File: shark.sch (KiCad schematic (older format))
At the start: 125 parts, among them J1 USB_B, SW1 MXSwitch, SW10 MXSwitch, SW11 MXSwitch, SW12 MXSwitch, SW13 MXSwitch, SW14 MXSwitch, SW15 MXSwitch, SW16 MXSwitch, SW17 MXSwitch, SW18 MXSwitch, SW19 MXSwitch, SW2 MXSwitch, SW20 MXSwitch, SW21 MXSwitch, SW22 MXSwitch, SW23 MXSwitch, SW24 MXSwitch, SW25 MXSwitch, SW26 MXSwitch, SW27 MXSwitch, SW28 MXSwitch, SW29 MXSwitch, SW3 MXSwitch, SW30 MXSwitch, SW31 MXSwitch, SW32 MXSwitch, SW33 MXSwitch, SW34 MXSwitch, SW35 MXSwitch, SW36 MXSwitch, SW37 MXSwitch, SW38 MXSwitch, SW39 MXSwitch, SW4 MXSwitch, SW40 MXSwitch, SW41 MXSwitch, SW42 MXSwitch, SW43 MXSwitch, SW44 MXSwitch, SW45 MXSwitch, SW46 MXSwitch, SW47 MXSwitch, SW48 MXSwitch, SW49 MXSwitch, SW5 MXSwitch, SW50 MXSwitch, SW51 MXSwitch, SW6 MXSwitch, SW7 MXSwitch, SW8 MXSwitch, SW9 MXSwitch, U1 ATmega32U4-AU, Y1 Crystal

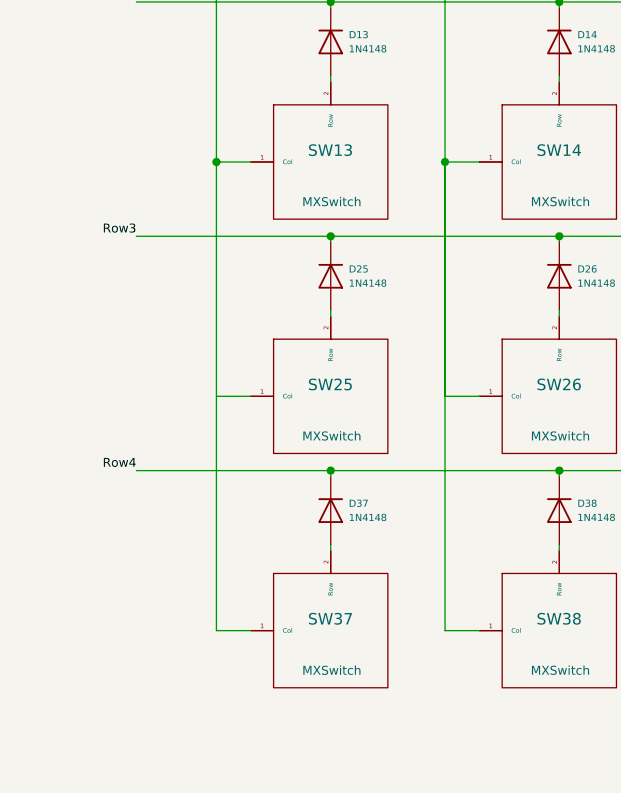
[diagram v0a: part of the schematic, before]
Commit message: Added row and column traces, fixed some components positions
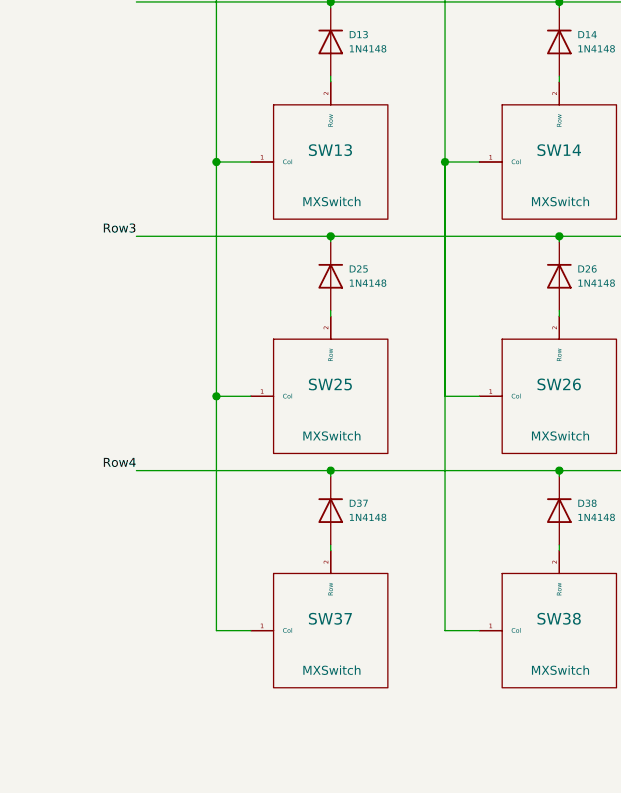
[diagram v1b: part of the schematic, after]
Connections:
- net Col1: now also SW25.1 (Col)
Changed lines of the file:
@@
 $EndComp
 Wire Wire Line
-	2150 3725 2150 5775
+	2150 3725 2150 4750
 Wire Wire Line
 	2150 2700 2150 3725
@@
 Wire Wire Line
 	6650 6100 6950 6100
+Connection ~ 2150 4750
+Wire Wire Line
+	2150 4750 2150 5775
 $EndSCHEMATC

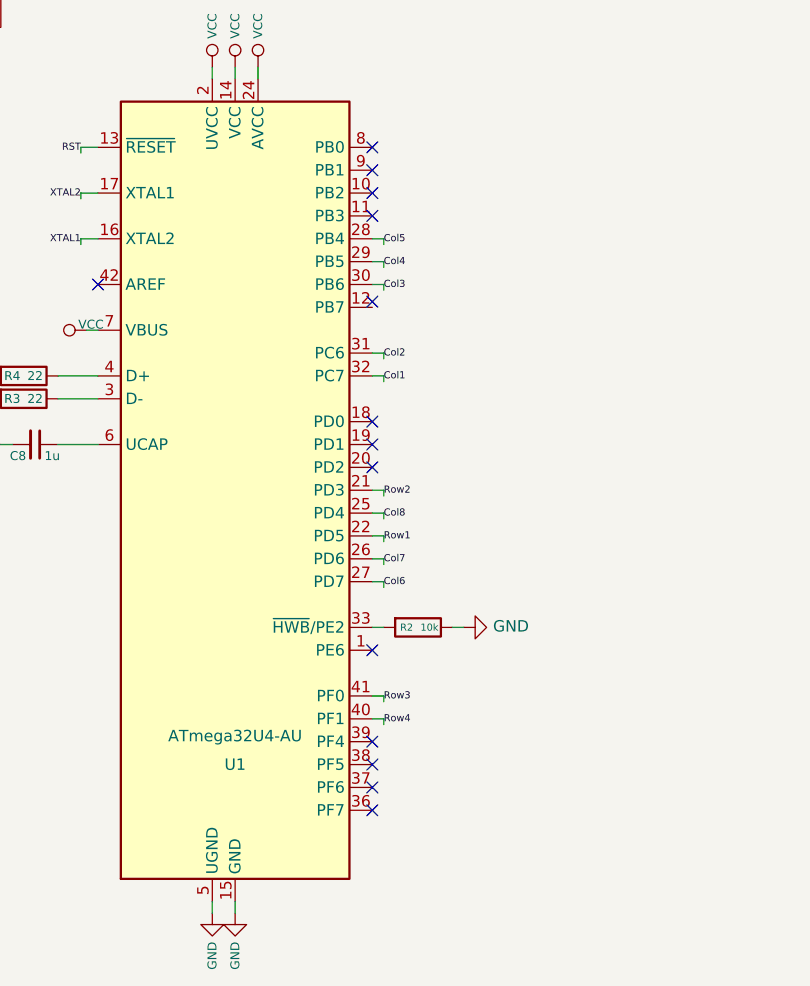
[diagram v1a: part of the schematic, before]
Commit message: Continued tracing
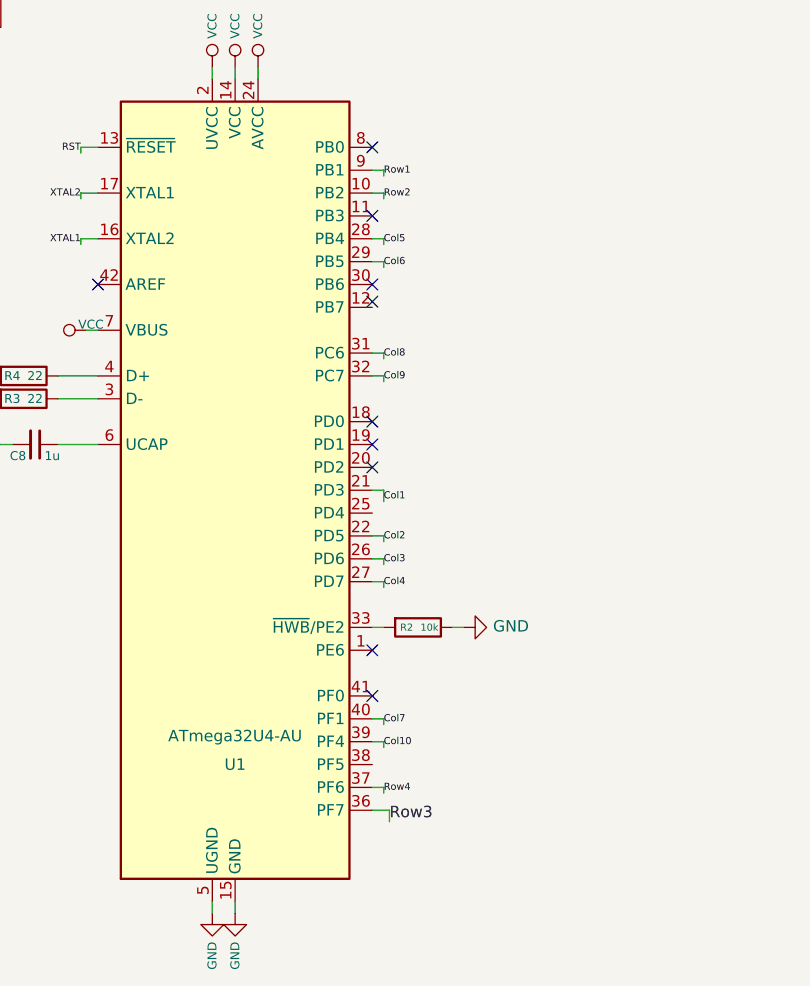
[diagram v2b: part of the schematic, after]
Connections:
- net Col1: now also U1.21 (PD3); no longer U1.32 (PC7)
- net Col10: now also U1.39 (PF4)
- net Col2: now also U1.22 (PD5); no longer U1.31 (PC6)
- net Col3: now also U1.26 (PD6); no longer U1.30 (PB6)
- net Col4: now also U1.27 (PD7); no longer U1.29 (PB5)
- net Col6: now also U1.29 (PB5); no longer U1.27 (PD7)
- net Col7: now also U1.40 (PF1); no longer U1.26 (PD6)
- net Col8: now also U1.31 (PC6); no longer U1.25 (PD4)
- net Col9: now also U1.32 (PC7)
- net Row1: now also U1.9 (PB1); no longer U1.22 (PD5)
- net Row2: now also U1.10 (PB2); no longer U1.21 (PD3)
- net Row3: now also U1.36 (PF7); no longer U1.41 (PF0)
- net Row4: now also U1.37 (PF6); no longer U1.40 (PF1)
- no-connect marks 14 -> 10
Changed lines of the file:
@@
 	10575 9400 10525 9400
-$Comp
-L power:GND #PWR0107
-U 1 1 5BEE37FA
-P 2125 8975
-F 0 "#PWR0107" H 2125 8725 50  0001 C CNN
-F 1 "GND" V 2130 8847 50  0000 R CNN
-F 2 "" H 2125 8975 50  0001 C CNN
-F 3 "" H 2125 8975 50  0001 C CNN
-	1    2125 8975
-	1    0    0    -1
-$EndComp
 $Comp
 L power:GND #PWR0108
@@
 Wire Wire Line
 	2225 8925 2225 9075
-Wire Wire Line
-	2125 8925 2125 8975
 $Comp
 L Device:R R3
@@
 	9250 7300 9325 7300
 Wire Wire Line
-	10525 8800 10575 8800
-Wire Wire Line
-	10525 9000 10575 9000
-Text Label 10575 8825 0    31   ~ 0
+	10525 7500 10575 7500
+Wire Wire Line
+	10525 7400 10575 7400
+Text Label 10575 7525 0    31   ~ 0
 Row2
-Text Label 10575 9025 0    31   ~ 0
+Text Label 10575 7425 0    31   ~ 0
 Row1
 Wire Wire Line
-	10525 8900 10575 8900
-Wire Wire Line
 	10525 9100 10575 9100
 Wire Wire Line
+	10525 9800 10575 9800
+Wire Wire Line
 	10525 9200 10575 9200
 Wire Wire Line
@@
 Wire Wire Line
 	10525 7800 10575 7800
-Wire Wire Line
-	10525 7900 10575 7900
-Text Label 10575 8925 0    31   ~ 0
-Col8
 Text Label 10575 9125 0    31   ~ 0
+Col3
+Text Label 10575 9825 0    31   ~ 0
 Col7
 Text Label 10575 9225 0    31   ~ 0
-Col6
+Col4
 Text Label 10575 7725 0    31   ~ 0
 Col5
 Text Label 10575 7825 0    31   ~ 0
-Col4
-Text Label 10575 7925 0    31   ~ 0
-Col3
-Wire Wire Line
-	10575 7925 10575 7900
+Col6
 Wire Wire Line
 	10575 7825 10575 7800
@@
 	10575 9200 10575 9225
 Wire Wire Line
+	10575 9800 10575 9825
+Wire Wire Line
 	10575 9100 10575 9125
-Wire Wire Line
-	10575 8900 10575 8925
 NoConn ~ 10525 9500
 Wire Wire Line
@@
 	10575 8300 10575 8325
 Text Label 10575 8325 0    31   ~ 0
-Col1
+Col9
 Text Label 10575 8225 0    31   ~ 0
-Col2
-Wire Wire Line
-	10525 9800 10575 9800
-Wire Wire Line
-	10575 9800 10575 9825
-Wire Wire Line
-	10525 9700 10575 9700
-Wire Wire Line
-	10575 9700 10575 9725
-Text Label 10575 9725 0    31   ~ 0
-Row3
-Text Label 10575 9825 0    31   ~ 0
+Col8
+Wire Wire Line
+	10525 10100 10575 10100
+Wire Wire Line
+	10575 10100 10575 10125
+Text Label 10575 10125 0    31   ~ 0
 Row4
 $Comp
@@
 $EndComp
 NoConn ~ 10525 7300
-NoConn ~ 10525 7400
-NoConn ~ 10525 7500
 NoConn ~ 10525 7600
 NoConn ~ 10525 7975
@@
 NoConn ~ 10525 8700
 Wire Wire Line
-	10575 9000 10575 9025
-Wire Wire Line
-	10575 8800 10575 8825
-NoConn ~ 10525 10200
-NoConn ~ 10525 10100
-NoConn ~ 10525 10000
-NoConn ~ 10525 9900
+	10575 7400 10575 7425
+Wire Wire Line
+	10575 7500 10575 7525
 NoConn ~ 9325 7900
 $Comp
@@
 Wire Wire Line
 	2150 4750 2150 5775
+Wire Wire Line
+	2125 8925 2125 8975
+$Comp
+L power:GND #PWR0107
+U 1 1 5BEE37FA
+P 2125 8975
+F 0 "#PWR0107" H 2125 8725 50  0001 C CNN
+F 1 "GND" V 2130 8847 50  0000 R CNN
+F 2 "" H 2125 8975 50  0001 C CNN
+F 3 "" H 2125 8975 50  0001 C CNN
+	1    2125 8975
+	1    0    0    -1
+$EndComp
+Wire Wire Line
+	10525 10200 10600 10200
+Wire Wire Line
+	10600 10200 10600 10250
+Text Label 10600 10250 0    50   ~ 0
+Row3
+NoConn ~ 10525 9700
+Wire Wire Line
+	10525 9900 10575 9900
+Wire Wire Line
+	10575 9900 10575 9925
+Text Label 10575 9925 0    31   ~ 0
+Col10
+NoConn ~ 10525 7900
+Wire Wire Line
+	10525 9000 10575 9000
+Text Label 10575 9025 0    31   ~ 0
+Col2
+Wire Wire Line
+	10575 9000 10575 9025
+Wire Wire Line
+	10525 8800 10575 8800
+Wire Wire Line
+	10575 8800 10575 8850
+Text Label 10575 8850 0    31   ~ 0
+Col1
 $EndSCHEMATC

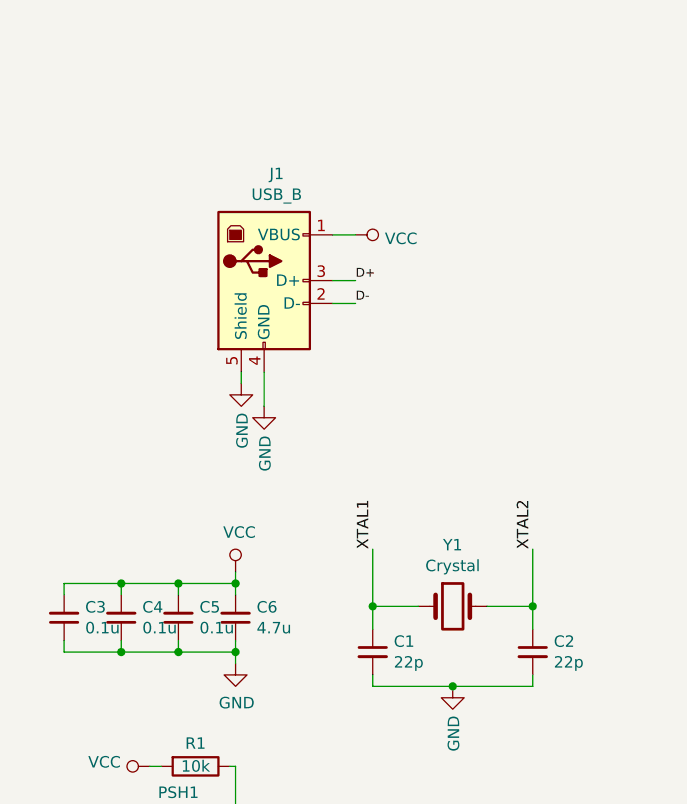
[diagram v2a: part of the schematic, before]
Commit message: Finished routing
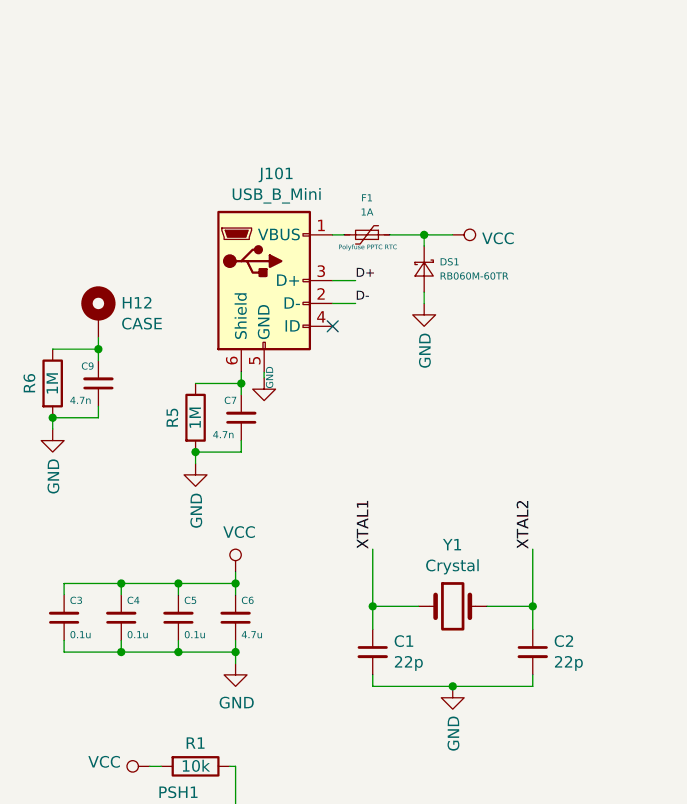
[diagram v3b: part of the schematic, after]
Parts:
- removed J1: USB_B, Connector_USB:USB_Micro-B_GCT_USB3076-30-A, symbol Connector:USB_B
- added C7, C9: 4.7n, Capacitor_SMD:C_0805_2012Metric_Pad1.15x1.40mm_HandSolder, symbol Device:C_Small
- added DS1: RB060M-60TR, Diode_SMD:D_SOD-123, symbol Device:D_Schottky_Small
- added F1: 1A, Fuse:Fuse_0805_2012Metric_Pad1.15x1.40mm_HandSolder, symbol Device:Polyfuse_Small
- added H12: CASE, Connector_Pin:Pin_D1.0mm_L10.0mm, symbol Mechanical:MountingHole_Pad
- added J101: USB_B_Mini, Keyboard_switches:miniB_connector, symbol Connector:USB_B_Mini
- added R5, R6: 1M, Resistor_SMD:R_1206_3216Metric_Pad1.42x1.75mm_HandSolder, symbol Device:R
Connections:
- net D+: now also J101.3 (D+)
- net D-: now also J101.2 (D-)
- net GND: now also C7.1, C9.1, DS1.2 (A), J101.5 (GND), R5.2, R6.2
- net VCC: now also DS1.1 (K), F1.1
- new net: C7.2, J101.6 (Shield), R5.1
- new net: F1.2, J101.1 (VBUS)
- new net: C9.2, H12.1, R6.1
- no-connect marks 10 -> 11
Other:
- note added: "Polyfuse PPTC RTC"
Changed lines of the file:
@@
 U 1 1 5BEDC719
 P 1350 10000
-F 0 "C3" H 1258 9954 50  0000 R CNN
-F 1 "0.1u" H 1258 10045 50  0000 R CNN
+F 0 "C3" H 1325 9925 31  0000 R CNN
+F 1 "0.1u" H 1325 10075 31  0000 R CNN
 F 2 "Capacitor_SMD:C_0805_2012Metric_Pad1.15x1.40mm_HandSolder" H 1350 10000 50  0001 C CNN
 F 3 "~" H 1350 10000 50  0001 C CNN
@@
 U 1 1 5BEDCA86
 P 1600 10000
-F 0 "C4" H 1508 9954 50  0000 R CNN
-F 1 "0.1u" H 1508 10045 50  0000 R CNN
+F 0 "C4" H 1575 9925 31  0000 R CNN
+F 1 "0.1u" H 1575 10075 31  0000 R CNN
 F 2 "Capacitor_SMD:C_0805_2012Metric_Pad1.15x1.40mm_HandSolder" H 1600 10000 50  0001 C CNN
 F 3 "~" H 1600 10000 50  0001 C CNN
@@
 U 1 1 5BEDCAA4
 P 1850 10000
-F 0 "C5" H 1758 9954 50  0000 R CNN
-F 1 "0.1u" H 1758 10045 50  0000 R CNN
+F 0 "C5" H 1825 9925 31  0000 R CNN
+F 1 "0.1u" H 1825 10075 31  0000 R CNN
 F 2 "Capacitor_SMD:C_0805_2012Metric_Pad1.15x1.40mm_HandSolder" H 1850 10000 50  0001 C CNN
 F 3 "~" H 1850 10000 50  0001 C CNN
@@
 U 1 1 5BEDCAC4
 P 2100 10000
-F 0 "C6" H 2008 9954 50  0000 R CNN
-F 1 "4.7u" H 2008 10045 50  0000 R CNN
+F 0 "C6" H 2075 9925 31  0000 R CNN
+F 1 "4.7u" H 2075 10075 31  0000 R CNN
 F 2 "Capacitor_SMD:C_0805_2012Metric_Pad1.15x1.40mm_HandSolder" H 2100 10000 50  0001 C CNN
 F 3 "~" H 2100 10000 50  0001 C CNN
@@
 L power:GND #PWR0108
 U 1 1 5BEE3841
-P 2225 9075
-F 0 "#PWR0108" H 2225 8825 50  0001 C CNN
-F 1 "GND" V 2230 8947 50  0000 R CNN
-F 2 "" H 2225 9075 50  0001 C CNN
-F 3 "" H 2225 9075 50  0001 C CNN
-	1    2225 9075
+P 2225 8950
+F 0 "#PWR0108" H 2225 8700 50  0001 C CNN
+F 1 "GND" V 2250 9000 31  0000 R CNN
+F 2 "" H 2225 8950 50  0001 C CNN
+F 3 "" H 2225 8950 50  0001 C CNN
+	1    2225 8950
 	1    0    0    -1
 $EndComp
@@
 Wire Wire Line
 	2625 8625 2525 8625
-Wire Wire Line
-	2625 8325 2525 8325
 $Comp
 L power:VCC #PWR0109
 U 1 1 5BEE4C80
-P 2625 8325
-F 0 "#PWR0109" H 2625 8175 50  0001 C CNN
-F 1 "VCC" V 2642 8453 50  0000 L CNN
-F 2 "" H 2625 8325 50  0001 C CNN
-F 3 "" H 2625 8325 50  0001 C CNN
-	1    2625 8325
+P 3050 8325
+F 0 "#PWR0109" H 3050 8175 50  0001 C CNN
+F 1 "VCC" V 3067 8453 50  0000 L CNN
+F 2 "" H 3050 8325 50  0001 C CNN
+F 3 "" H 3050 8325 50  0001 C CNN
+	1    3050 8325
 	0    1    1    0
 $EndComp
@@
 D+
 Wire Wire Line
-	2225 8925 2225 9075
+	2225 8925 2225 8950
 $Comp
 L Device:R R3
@@
 NoConn ~ 9325 7900
 $Comp
-L Connector:USB_B J1
-U 1 1 5CE1CB19
-P 2225 8525
-F 0 "J1" H 2280 8992 50  0000 C CNN
-F 1 "USB_B" H 2280 8901 50  0000 C CNN
-F 2 "Connector_USB:USB_Micro-B_GCT_USB3076-30-A" H 2375 8475 50  0001 C CNN
-F 3 " ~" H 2375 8475 50  0001 C CNN
-	1    2225 8525
-	1    0    0    -1
-$EndComp
-$Comp
 L Device:Crystal Y1
 U 1 1 5CF9FC7C
@@
 Wire Wire Line
 	2125 8925 2125 8975
-$Comp
-L power:GND #PWR0107
-U 1 1 5BEE37FA
-P 2125 8975
-F 0 "#PWR0107" H 2125 8725 50  0001 C CNN
-F 1 "GND" V 2130 8847 50  0000 R CNN
-F 2 "" H 2125 8975 50  0001 C CNN
-F 3 "" H 2125 8975 50  0001 C CNN
-	1    2125 8975
-	1    0    0    -1
-$EndComp
 Wire Wire Line
 	10525 10200 10600 10200
@@
 Text Label 10575 8850 0    31   ~ 0
 Col1
+$Comp
+L Device:C_Small C7
+U 1 1 5C192852
+P 2125 9125
+F 0 "C7" H 2200 9050 31  0000 R CNN
+F 1 "4.7n" H 2250 9200 31  0000 R CNN
+F 2 "Capacitor_SMD:C_0805_2012Metric_Pad1.15x1.40mm_HandSolder" H 2125 9125 50  0001 C CNN
+F 3 "~" H 2125 9125 50  0001 C CNN
+	1    2125 9125
+	-1   0    0    1
+$EndComp
+$Comp
+L Device:R R5
+U 1 1 5C1953C2
+P 1925 9125
+F 0 "R5" V 1825 9125 50  0000 C CNN
+F 1 "1M" V 1925 9125 50  0000 C CNN
+F 2 "Resistor_SMD:R_1206_3216Metric_Pad1.42x1.75mm_HandSolder" V 1855 9125 50  0001 C CNN
+F 3 "~" H 1925 9125 50  0001 C CNN
+	1    1925 9125
+	1    0    0    -1
+$EndComp
+Wire Wire Line
+	1925 8975 2125 8975
+Wire Wire Line
+	2125 8975 2125 9025
+Connection ~ 2125 8975
+Wire Wire Line
+	2125 9225 2125 9275
+Wire Wire Line
+	2125 9275 1925 9275
+Wire Wire Line
+	1925 9275 1925 9325
+Connection ~ 1925 9275
+$Comp
+L power:GND #PWR0107
+U 1 1 5C237223
+P 1925 9325
+F 0 "#PWR0107" H 1925 9075 50  0001 C CNN
+F 1 "GND" V 1930 9197 50  0000 R CNN
+F 2 "" H 1925 9325 50  0001 C CNN
+F 3 "" H 1925 9325 50  0001 C CNN
+	1    1925 9325
+	1    0    0    -1
+$EndComp
+$Comp
+L Device:Polyfuse_Small F1
+U 1 1 5C25B88F
+P 2675 8325
+F 0 "F1" V 2514 8325 31  0000 C CNN
+F 1 "1A" V 2576 8325 31  0000 C CNN
+F 2 "Fuse:Fuse_0805_2012Metric_Pad1.15x1.40mm_HandSolder" H 2725 8125 50  0001 L CNN
+F 3 "~" H 2675 8325 50  0001 C CNN
+	1    2675 8325
+	0    1    1    0
+$EndComp
+Wire Wire Line
+	2525 8325 2575 8325
+Text Notes 2550 8400 0    20   ~ 0
+Polyfuse PPTC RTC
+$Comp
+L Device:D_Schottky_Small DS1
+U 1 1 5C2FFE6A
+P 2925 8475
+F 0 "DS1" V 2894 8543 31  0000 L CNN
+F 1 "RB060M-60TR" V 2956 8543 31  0000 L CNN
+F 2 "Diode_SMD:D_SOD-123" V 2925 8475 50  0001 C CNN
+F 3 "~" V 2925 8475 50  0001 C CNN
+	1    2925 8475
+	0    1    1    0
+$EndComp
+Wire Wire Line
+	2775 8325 2925 8325
+Wire Wire Line
+	2925 8325 2925 8375
+Connection ~ 2925 8325
+Wire Wire Line
+	2925 8325 3050 8325
+Wire Wire Line
+	2925 8575 2925 8625
+$Comp
+L power:GND #PWR0112
+U 1 1 5C363806
+P 2925 8625
+F 0 "#PWR0112" H 2925 8375 50  0001 C CNN
+F 1 "GND" V 2930 8497 50  0000 R CNN
+F 2 "" H 2925 8625 50  0001 C CNN
+F 3 "" H 2925 8625 50  0001 C CNN
+	1    2925 8625
+	1    0    0    -1
+$EndComp
+$Comp
+L Connector:USB_B_Mini J101
+U 1 1 5C3661B8
+P 2225 8525
+F 0 "J101" H 2280 8992 50  0000 C CNN
+F 1 "USB_B_Mini" H 2280 8901 50  0000 C CNN
+F 2 "Keyboard_switches:miniB_connector" H 2375 8475 50  0001 C CNN
+F 3 "~" H 2375 8475 50  0001 C CNN
+	1    2225 8525
+	1    0    0    -1
+$EndComp
+NoConn ~ 2525 8725
+Wire Wire Line
+	1500 8775 1500 8825
+$Comp
+L Device:C_Small C9
+U 1 1 5C391EB2
+P 1500 8975
+F 0 "C9" H 1575 8900 31  0000 R CNN
+F 1 "4.7n" H 1625 9050 31  0000 R CNN
+F 2 "Capacitor_SMD:C_0805_2012Metric_Pad1.15x1.40mm_HandSolder" H 1500 8975 50  0001 C CNN
+F 3 "~" H 1500 8975 50  0001 C CNN
+	1    1500 8975
+	-1   0    0    1
+$EndComp
+$Comp
+L Device:R R6
+U 1 1 5C391EB9
+P 1300 8975
+F 0 "R6" V 1200 8975 50  0000 C CNN
+F 1 "1M" V 1300 8975 50  0000 C CNN
+F 2 "Resistor_SMD:R_1206_3216Metric_Pad1.42x1.75mm_HandSolder" V 1230 8975 50  0001 C CNN
+F 3 "~" H 1300 8975 50  0001 C CNN
+	1    1300 8975
+	1    0    0    -1
+$EndComp
+Wire Wire Line
+	1300 8825 1500 8825
+Wire Wire Line
+	1500 8825 1500 8875
+Connection ~ 1500 8825
+Wire Wire Line
+	1500 9075 1500 9125
+Wire Wire Line
+	1500 9125 1300 9125
+Wire Wire Line
+	1300 9125 1300 9175
+Connection ~ 1300 9125
+$Comp
+L power:GND #PWR0113
+U 1 1 5C391EC7
+P 1300 9175
+F 0 "#PWR0113" H 1300 8925 50  0001 C CNN
+F 1 "GND" V 1305 9047 50  0000 R CNN
+F 2 "" H 1300 9175 50  0001 C CNN
+F 3 "" H 1300 9175 50  0001 C CNN
+	1    1300 9175
+	1    0    0    -1
+$EndComp
+$Comp
+L Mechanical:MountingHole_Pad H12
+U 1 1 5C3B52F4
+P 1500 8675
+F 0 "H12" H 1600 8726 50  0000 L CNN
+F 1 "CASE" H 1600 8635 50  0000 L CNN
+F 2 "Connector_Pin:Pin_D1.0mm_L10.0mm" H 1500 8675 50  0001 C CNN
+F 3 "~" H 1500 8675 50  0001 C CNN
+	1    1500 8675
+	1    0    0    -1
+$EndComp
 $EndSCHEMATC

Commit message: Fixed schematic, removed stitches
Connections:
- net Col7: now also U1.19 (PD1); no longer U1.40 (PF1)
- net Col8: now also U1.18 (PD0); no longer U1.31 (PC6)
- net XTAL1: now also C2.1, U1.17 (XTAL1), Y1.2; no longer C1.1, U1.16 (XTAL2), Y1.1
- net XTAL2: now also C1.1, U1.16 (XTAL2), Y1.1; no longer C2.1, U1.17 (XTAL1), Y1.2
- no-connect marks 11 -> 13
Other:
- moved on the sheet: C1, C2, C3, C4, C5, C6, C7, C8, C9, D1, D10, D11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
